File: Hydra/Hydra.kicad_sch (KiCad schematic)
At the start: 116 parts, among them J1 USB_C_Receptacle_USB2.0, SW1 SW_Push, U1 USBLC6-2SC6, U2 ATmega32U4-M, Y1 16MHz

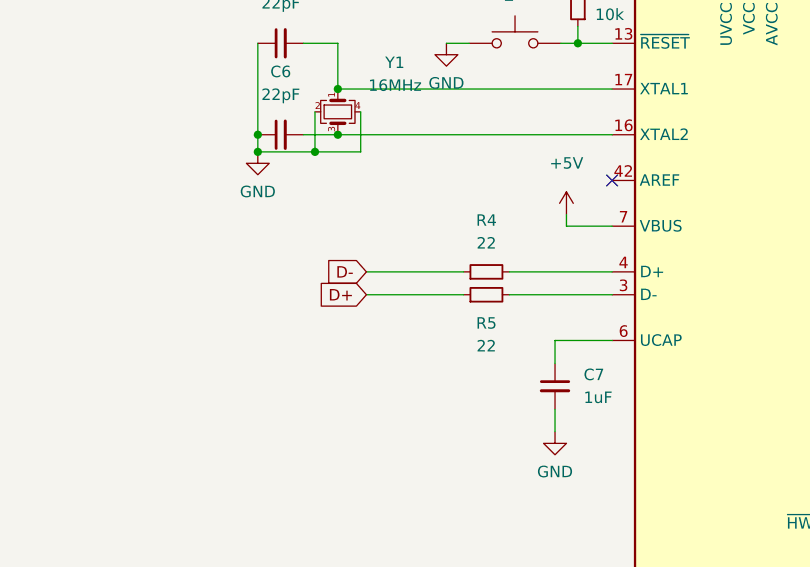
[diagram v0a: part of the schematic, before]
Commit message: mcu traces
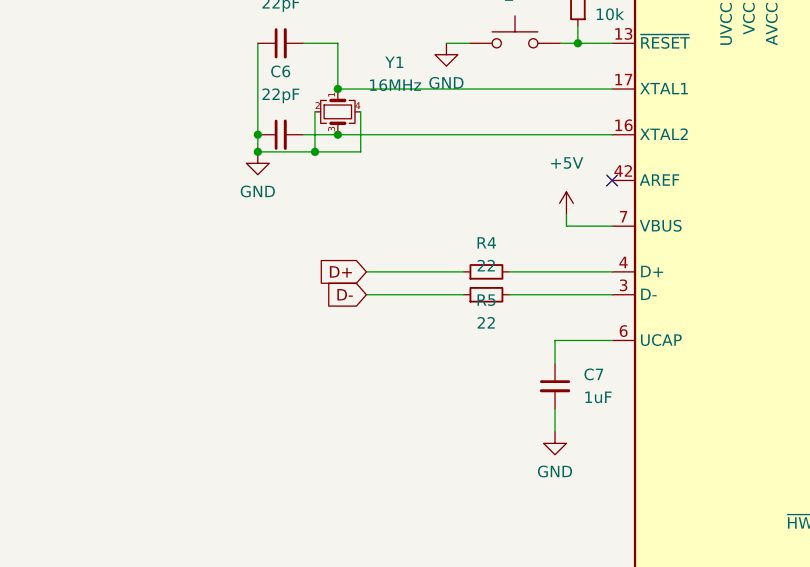
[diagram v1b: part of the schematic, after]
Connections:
- net at R4.2: now also U2.3 (D-); no longer U2.4 (D+)
- net at R5.2: now also U2.4 (D+); no longer U2.3 (D-)
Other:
- moved on the sheet: R4, R5
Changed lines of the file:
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@@
     )
   )
-  (global_label "D+" (shape input) (at 194.31 59.055 180) (fields_autoplaced)
+  (global_label "D+" (shape input) (at 194.31 56.515 180) (fields_autoplaced)
     (effects (font (size 1.27 1.27)) (justify right))
-    (property "Intersheet References" "${INTERSHEET_REFS}" (id 0) (at 189.0545 59.1344 0)
+    (property "Intersheet References" "${INTERSHEET_REFS}" (id 0) (at 189.0545 56.5944 0)
       (effects (font (size 1.27 1.27)) (justify right) hide)
     )
@@
     )
   )
-  (global_label "D-" (shape input) (at 194.31 56.515 180) (fields_autoplaced)
+  (global_label "D-" (shape input) (at 194.31 59.055 180) (fields_autoplaced)
     (effects (font (size 1.27 1.27)) (justify right))
-    (property "Intersheet References" "${INTERSHEET_REFS}" (id 0) (at 189.0545 56.4356 0)
+    (property "Intersheet References" "${INTERSHEET_REFS}" (id 0) (at 189.0545 58.9756 0)
       (effects (font (size 1.27 1.27)) (justify right) hide)
     )
@@
     (pin "2")
   )
-  (symbol (lib_id "Device:R_Small") (at 207.645 56.515 90) (unit 1)
-    (in_bom yes) (on_board yes) (fields_autoplaced)
-    (property "Reference" "R4" (id 0) (at 207.645 50.8 90))
-    (property "Value" "22" (id 1) (at 207.645 53.34 90))
-    (property "Footprint" "Resistor_SMD:R_0805_2012Metric" (id 2) (at 207.645 56.515 0)
-      (effects (font (size 1.27 1.27)) hide)
-    )
-    (property "Datasheet" "~" (id 3) (at 207.645 56.515 0)
+  (symbol (lib_id "Device:R_Small") (at 207.645 59.055 90) (unit 1)
+    (in_bom yes) (on_board yes) (fields_autoplaced)
+    (property "Reference" "R4" (id 0) (at 207.645 53.34 90))
+    (property "Value" "22" (id 1) (at 207.645 55.88 90))
+    (property "Footprint" "Resistor_SMD:R_0805_2012Metric" (id 2) (at 207.645 59.055 0)
+      (effects (font (size 1.27 1.27)) hide)
+    )
+    (property "Datasheet" "~" (id 3) (at 207.645 59.055 0)
       (effects (font (size 1.27 1.27)) hide)
     )
@@
     (pin "2")
   )
-  (symbol (lib_id "Device:R_Small") (at 207.645 59.055 90) (unit 1)
+  (symbol (lib_id "Device:R_Small") (at 207.645 56.515 90) (unit 1)
     (in_bom yes) (on_board yes)
-    (property "Reference" "R5" (id 0) (at 207.645 62.23 90))
-    (property "Value" "22" (id 1) (at 207.645 64.77 90))
-    (property "Footprint" "Resistor_SMD:R_0805_2012Metric" (id 2) (at 207.645 59.055 0)
-      (effects (font (size 1.27 1.27)) hide)
-    )
-    (property "Datasheet" "~" (id 3) (at 207.645 59.055 0)
-      (effects (font (size 1.27 1.27)) hide)
-    )
+    (property "Reference" "R5" (id 0) (at 207.645 59.69 90))
+    (property "Value" "22" (id 1) (at 207.645 62.23 90))
+    (property "Footprint" "Resistor_SMD:R_0805_2012Metric" (id 2) (at 207.645 56.515 0)
+      (effects (font (size 1.27 1.27)) hide)
+    )
+    (property "Datasheet" "~" (id 3) (at 207.645 56.515 0)
+      (effects (font (size 1.27 1.27)) hide)
+    )
